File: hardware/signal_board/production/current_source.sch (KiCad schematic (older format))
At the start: 35 parts, among them Q10 Q_PMOS_GDS, Q11 Q_NMOS_GDS, Q12 Q_NMOS_GSD, Q8 Q_NMOS_GSD, Q9 Q_NMOS_GSD, U4 LM324, U5 MCP6001-OT

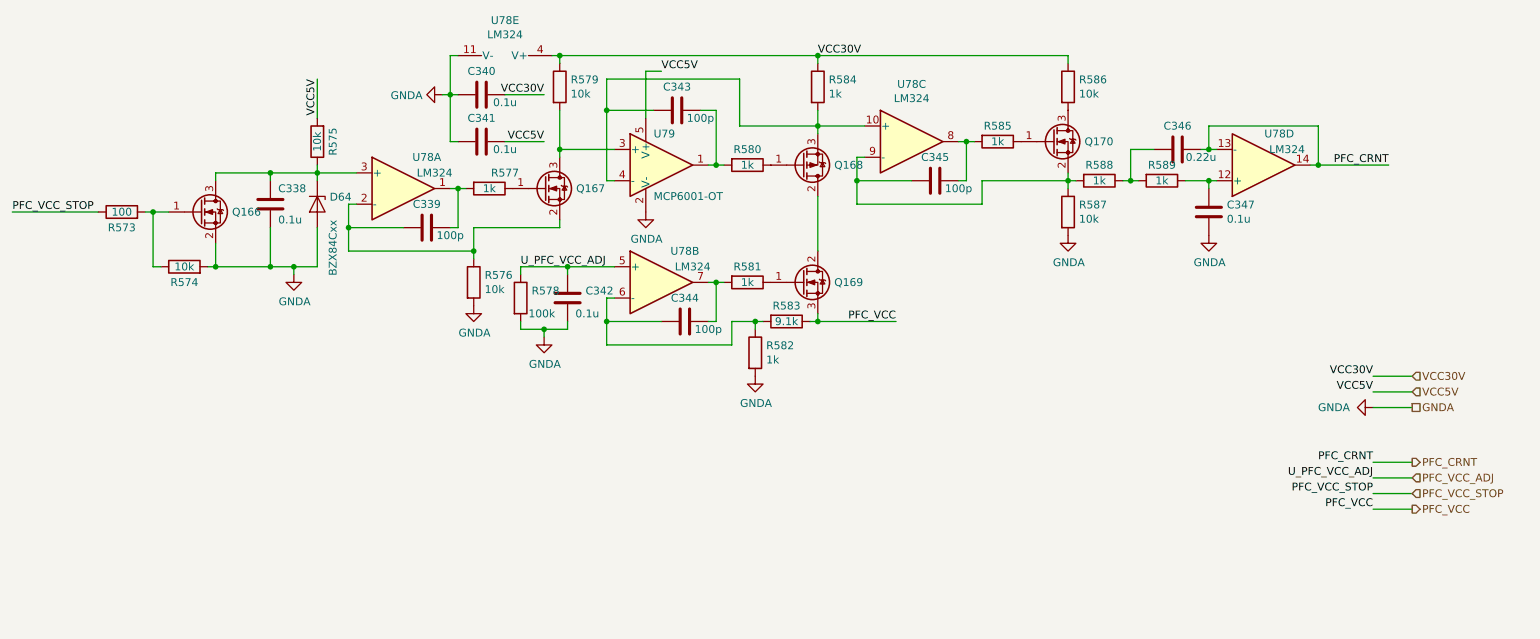
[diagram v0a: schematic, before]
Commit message: fix
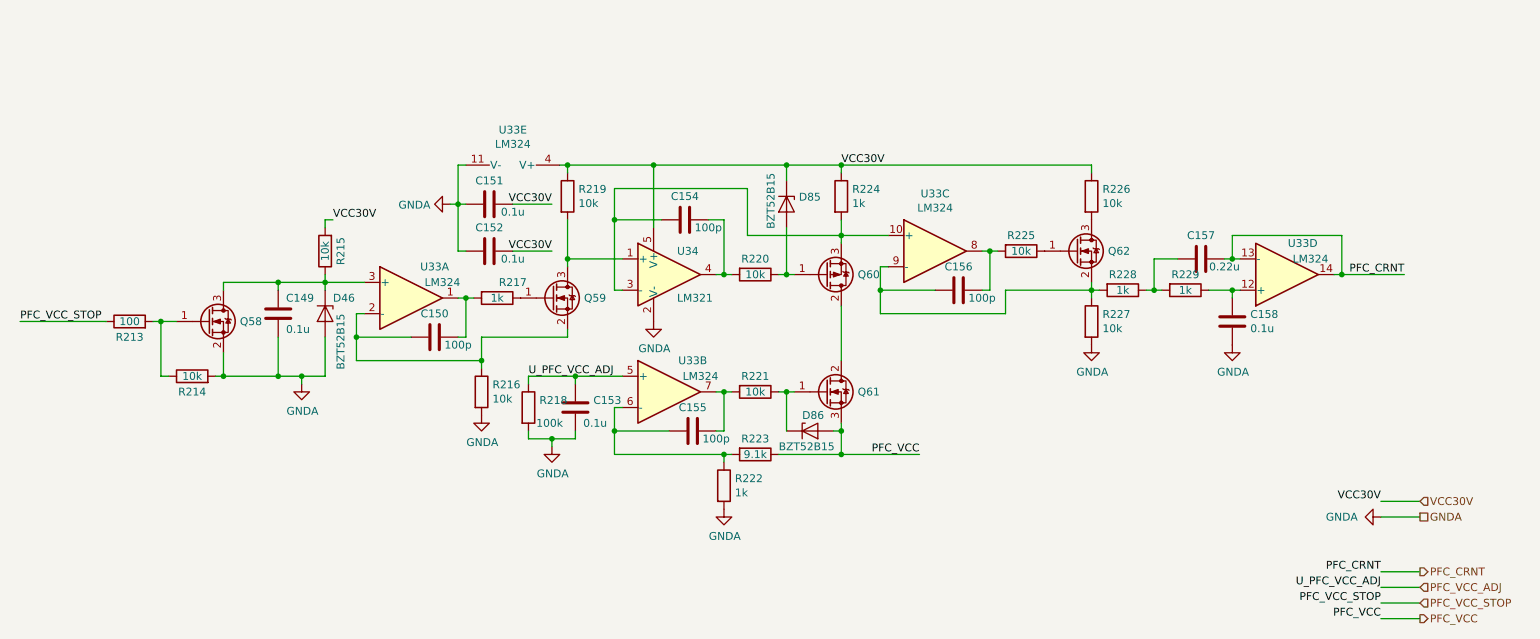
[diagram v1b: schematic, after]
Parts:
- removed D2: BZX84Cxx, Diode_SMD:D_SOT-23_ANK, symbol Diode:BZX84Cxx
- removed U5: MCP6001-OT, Package_TO_SOT_SMD:SOT-23-5, symbol Amplifier_Operational:MCP6001-OT
- added D2, D69, D70: BZT52B15, Diode_SMD:D_SOD-123, symbol Diode:BZT52Bxx
- added U5: LM321, Package_TO_SOT_SMD:SOT-23-5, symbol Amplifier_Operational:LM321
- R31, R32, R36: value 1k -> 10k
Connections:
- net VCC5V is gone; now on net VCC30V: C15.1, R26.2
- net GNDA: now also D2.2 (A), U5.2 (V-)
- net PFC_VCC: now also D70.2 (A)
- net VCC30V: now also D69.1 (K), U5.5 (V+)
- net at C12.1, Q8.3 (D), R26.1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: now also D2.1 (K)
- net at C17.2, Q10.3 (S), R35.2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: now also U5.3 (-)
- net at Q9.3 (D), R30.2: now also U5.1 (+)
- net at Q10.1 (G), R31.1: now also D69.2 (A)
- net at C17.1, R31.2: now also U5.4
- net at Q11.1 (G), R32.1: now also D70.1 (K)
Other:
- moved on the sheet: C149, C150, C151, C152, C153, C154, C155, C156, C157, C158, Q58, Q59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
